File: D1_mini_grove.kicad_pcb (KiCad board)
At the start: 2 copper layers, 25.7 x 34.3 mm, 9 parts, among them P1 Connector_Generic:Conn_01x08, P2 Connector_Generic:Conn_01x08

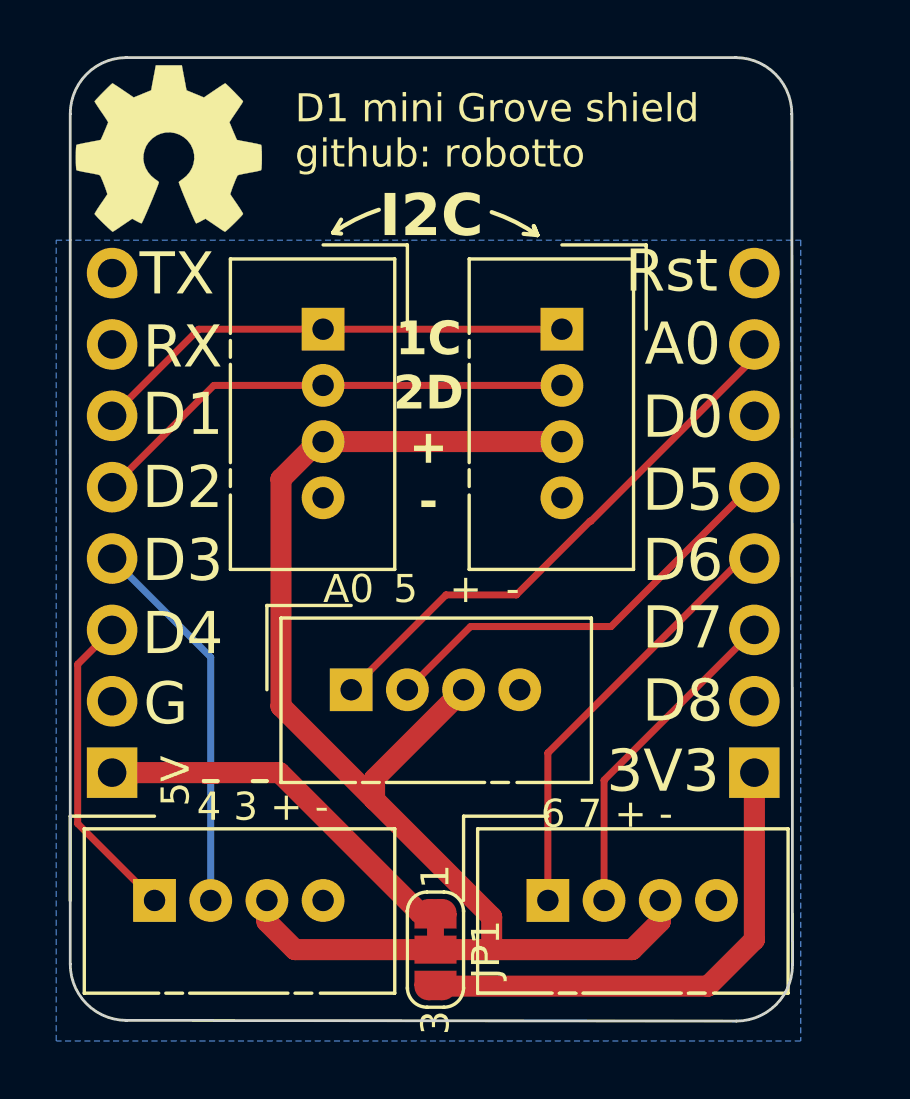
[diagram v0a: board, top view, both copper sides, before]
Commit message: flipped some stuff around
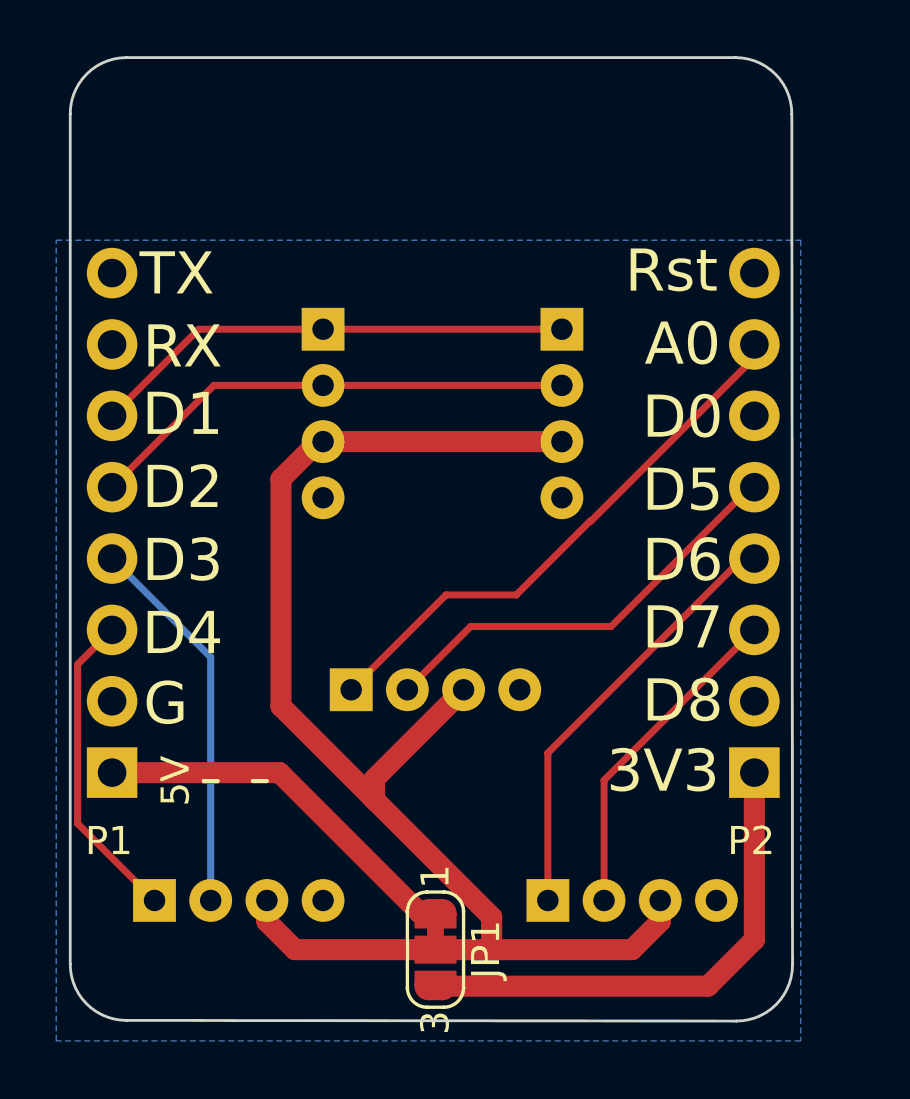
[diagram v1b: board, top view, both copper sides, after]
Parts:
- 1_2_IIC1, 1_2_IIC2, 3_4, 5_6, A0_7, REF**: moved to B.Cu
- P1, P2: moved to F.Cu
- moved REF** 18.4 mm to (147.9, 81.8), turned to 180 degrees
- turned 1_2_IIC1 to 180 degrees
- turned 1_2_IIC2 to 180 degrees
- turned 3_4 to -90 degrees
- turned 5_6 to -90 degrees
- turned A0_7 to -90 degrees
- turned P1 to 180 degrees
- turned P2 to 180 degrees
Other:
- board text added: "- + 3 4"
- board text added: "- + 7 6"
- board text removed: "4 3 + -"
- board text removed: "6 7 + -"
